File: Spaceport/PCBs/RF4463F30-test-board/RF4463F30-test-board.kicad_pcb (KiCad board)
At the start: 2 copper layers, 57.6 x 62.1 mm, 17 parts

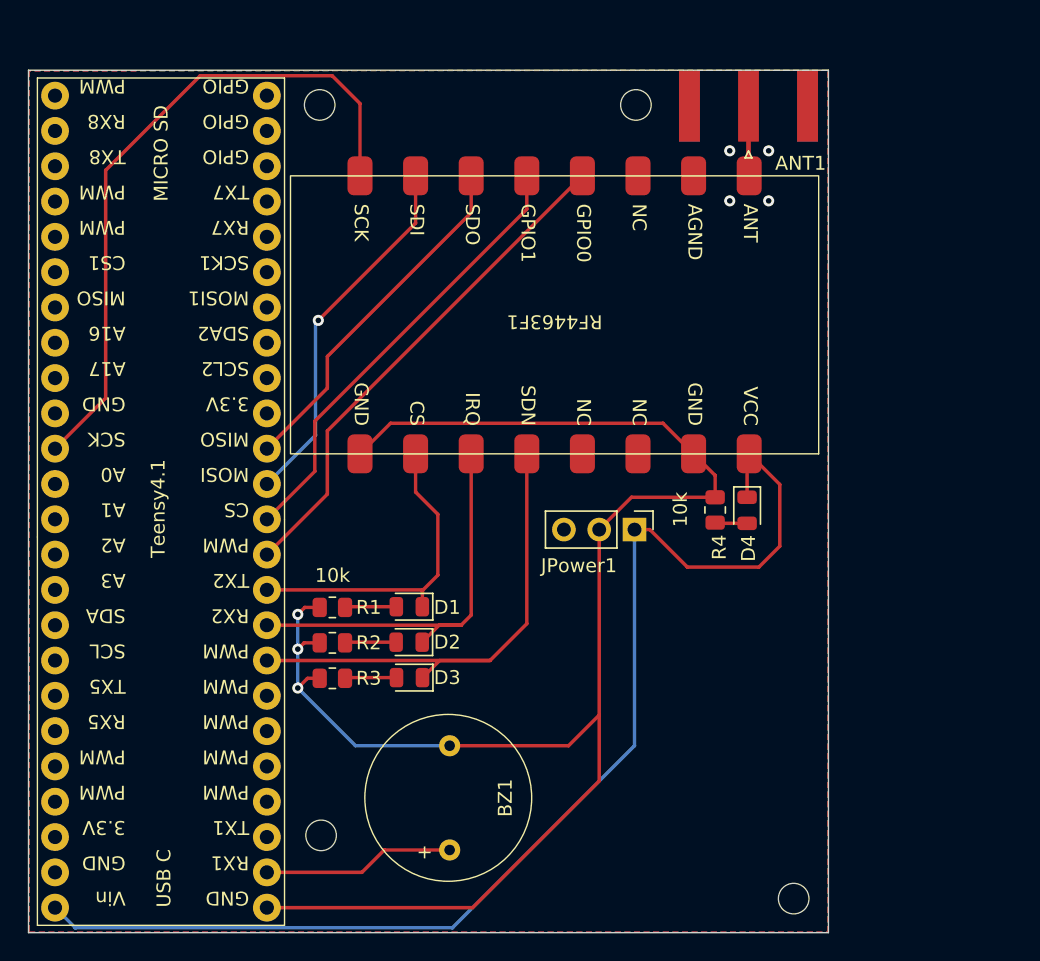
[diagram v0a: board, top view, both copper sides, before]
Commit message: initial COTS board updates
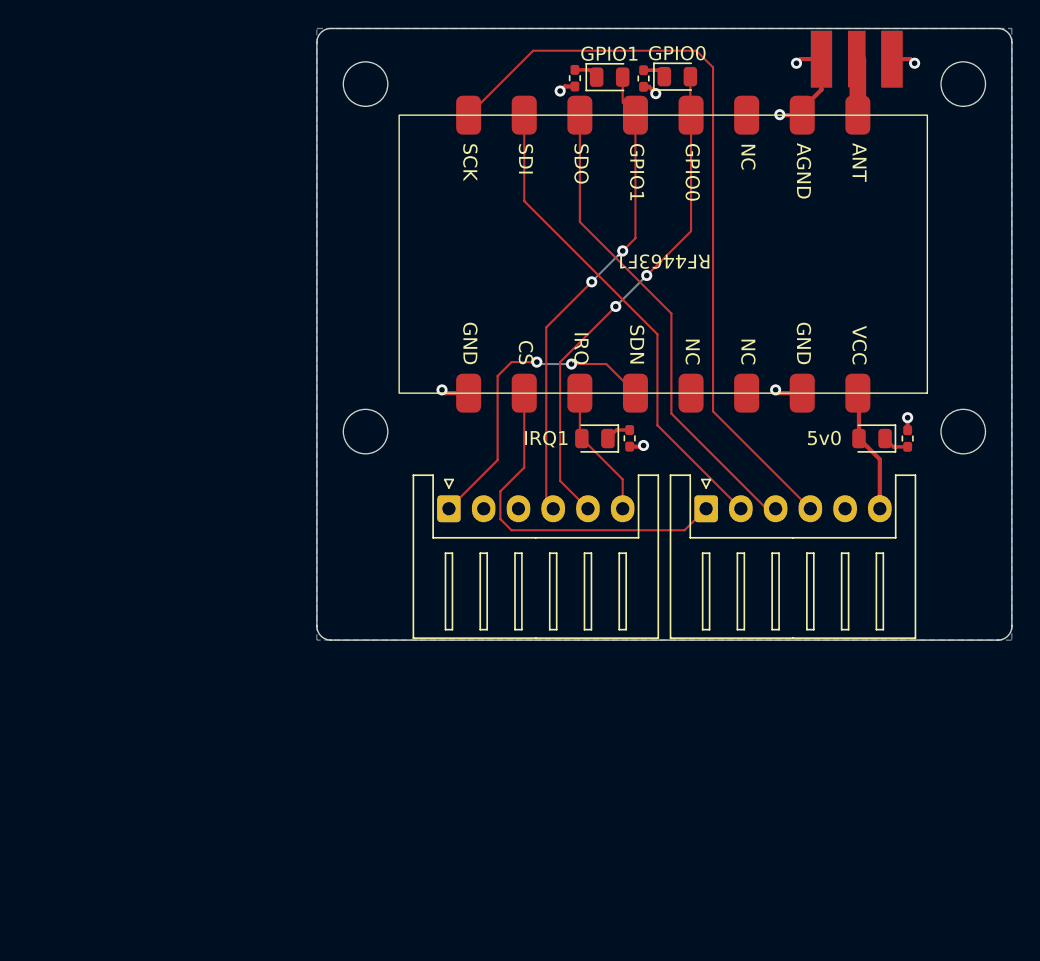
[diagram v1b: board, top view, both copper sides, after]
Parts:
- removed BZ1: Buzzer, Avionics:Adafruit_5V_Buzzer
- removed D1, D2, D3, D4: LED, LED_SMD:LED_0805_2012Metric
- removed JPower1: Conn_01x03_Pin, Connector_PinHeader_2.54mm:PinHeader_1x03_P2.54mm_Vertical
- removed Teensy4.1: ~, Avionics:Teensy_4.1
- added 5v0: LED, LED_SMD:LED_0805_2012Metric, F.Cu at (176.4, 103.5)
- added G***: LOGO, Avionics:LOGO, B.Cu at (168.5, 89.9)
- added GPIO0: LED, LED_SMD:LED_0805_2012Metric, F.Cu at (162.4, 77.5)
- added GPIO1: LED, LED_SMD:LED_0805_2012Metric, F.Cu at (157.6, 77.5)
- added IRQ1: LED, LED_SMD:LED_0805_2012Metric, F.Cu at (156.5, 103.5)
- added J1: Conn_01x06_Pin, Connector_JST:JST_XH_S6B-XH-A_1x06_P2.50mm_Horizontal, F.Cu at (164.5, 108.5)
- added J2: Conn_01x06_Pin, Connector_JST:JST_XH_S6B-XH-A_1x06_P2.50mm_Horizontal, F.Cu at (146.0, 108.5)
- ANT1: footprint Connector_Coaxial:SMA_Amphenol_132289_EdgeMount -> adafruit:SMA_EDGELAUNCH
- H1, H2, H3, H4: footprint MountingHole:MountingHole_2.2mm_M2 -> MountingHole:MountingHole_3.2mm_M3
- R1, R2, R3, R4: value 10k -> 5.1k; footprint Resistor_SMD:R_0805_2012Metric -> Resistor_SMD:R_0402_1005Metric_Pad0.72x0.64mm_HandSolder
- moved H4 54.1 mm to (140.0, 78.0), turned to 180 degrees
- moved R3 48.6 mm to (160.0, 77.6), turned to -90 degrees
- moved H3 46.3 mm to (183.0, 78.0), turned to 180 degrees
- moved H2 45.6 mm to (140.0, 103.0), turned to 180 degrees
- moved R2 44.2 mm to (155.1, 77.6), turned to -90 degrees
- moved H1 33.3 mm to (183.0, 103.0), turned to 180 degrees
- moved R1 24.6 mm to (159.0, 103.5), turned to -90 degrees
- moved R4 14.8 mm to (179.0, 103.5)
- moved ANT1 9.50 mm to (175.3, 74.2), turned to -90 degrees
- moved RF4463F1 8.95 mm to (161.4, 90.2)
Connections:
- ANT1 pad 2: Net-(ANT1-Ext) -> GND
- R1 pad 2: /GND -> GND
- R2 pad 2: /GND -> GND
- R3 pad 2: /GND -> GND
- R4 pad 2: /GND -> GND
- RF4463F1 pad 1: /5V -> +5V
- RF4463F1 pad 10: /MOSI -> MOSI
- RF4463F1 pad 11: /MISO -> MISO
- RF4463F1 pad 12: /GPIO1 -> GPIO1
- RF4463F1 pad 13: /GPIO0 -> GPIO0
- RF4463F1 pad 15: Net-(ANT1-Ext) -> GND
- RF4463F1 pad 2: /GND -> GND
- RF4463F1 pad 5: /SDN -> SDN
- RF4463F1 pad 6: /IRQ -> IRQ
- RF4463F1 pad 7: /CS -> CS
- RF4463F1 pad 8: /GND -> GND
- RF4463F1 pad 9: /SCK -> SCK
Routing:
- net /GND: track 119.7 -> 0.00 mm, vias 3 -> 0
- net /5V: track 86.2 -> 0.00 mm
- net SCK: track 0.00 -> 54.6 mm
- net /SCK: track 48.7 -> 0.00 mm
- net /SDN: track 37.3 -> 0.00 mm
- net /GPIO0: track 37.2 -> 0.00 mm
- net GPIO0: track 0.00 -> 35.8 mm, vias 0 -> 2
- net MOSI: track 0.00 -> 34.8 mm
- net MISO: track 0.00 -> 34.5 mm
- net GPIO1: track 0.00 -> 34.3 mm, vias 0 -> 2
- net /GPIO1: track 32.5 -> 0.00 mm
- net /IRQ: track 29.9 -> 0.00 mm
- net /MOSI: track 26.6 -> 0.00 mm, vias 1 -> 0
- net /MISO: track 25.7 -> 0.00 mm
- net CS: track 0.00 -> 25.5 mm
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- added copper zone on B.Cu, net GND
- removed copper zone on B.Cu, net Net-(ANT1-Ext)
- removed copper zone on F.Cu, net Net-(ANT1-Ext)
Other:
- board size 57.6 x 62.1 mm -> 50 x 44 mm
- board text added: "COTS Board v2"
